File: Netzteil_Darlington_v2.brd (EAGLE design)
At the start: 141 x 115.5 mm, 169 parts, among them IC1 NCP718BSN330T1G, IC10 LT4320DIL08, IC11 OPA2197, IC12 REF5040, IC13 OPA2197, IC15 LD33V, IC17 7818TV, IC18 ADS1015, IC19 ADS1015, IC2 OPA2197, IC3 DAC8311, IC4 VXO78012-1000, IC5 7815TV, IC6 VXO7805-1000, IC7 DAC8311, IC8 LTC6102HMS8#PBF, IC9 NCP718BSN330T1G, T1 IRLL110TRPBF, T10 BC847ALT1G, T11 BC847ALT1G, T12 DMG2302UK-7, T13 DMG2302UK-7, T14 DMG2302UK-7, T2 BC847ALT1G, T3 BD139, T4 DMMT5551-7-F, T5 TIP3055, T6 TIP3055, T7 BD139

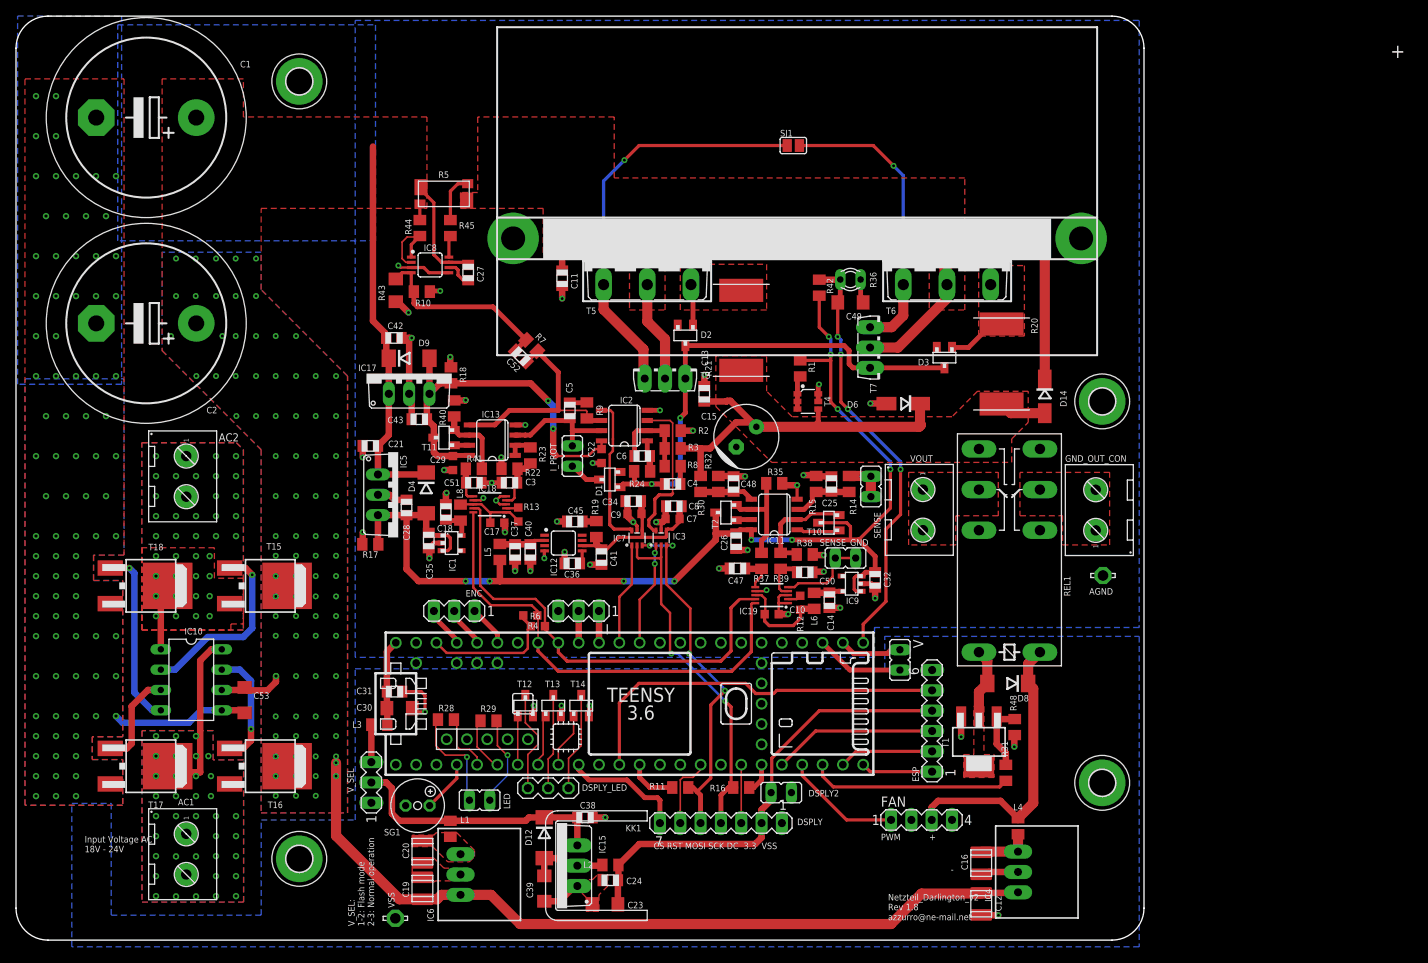
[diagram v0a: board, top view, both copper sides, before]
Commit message: Update to v1.9
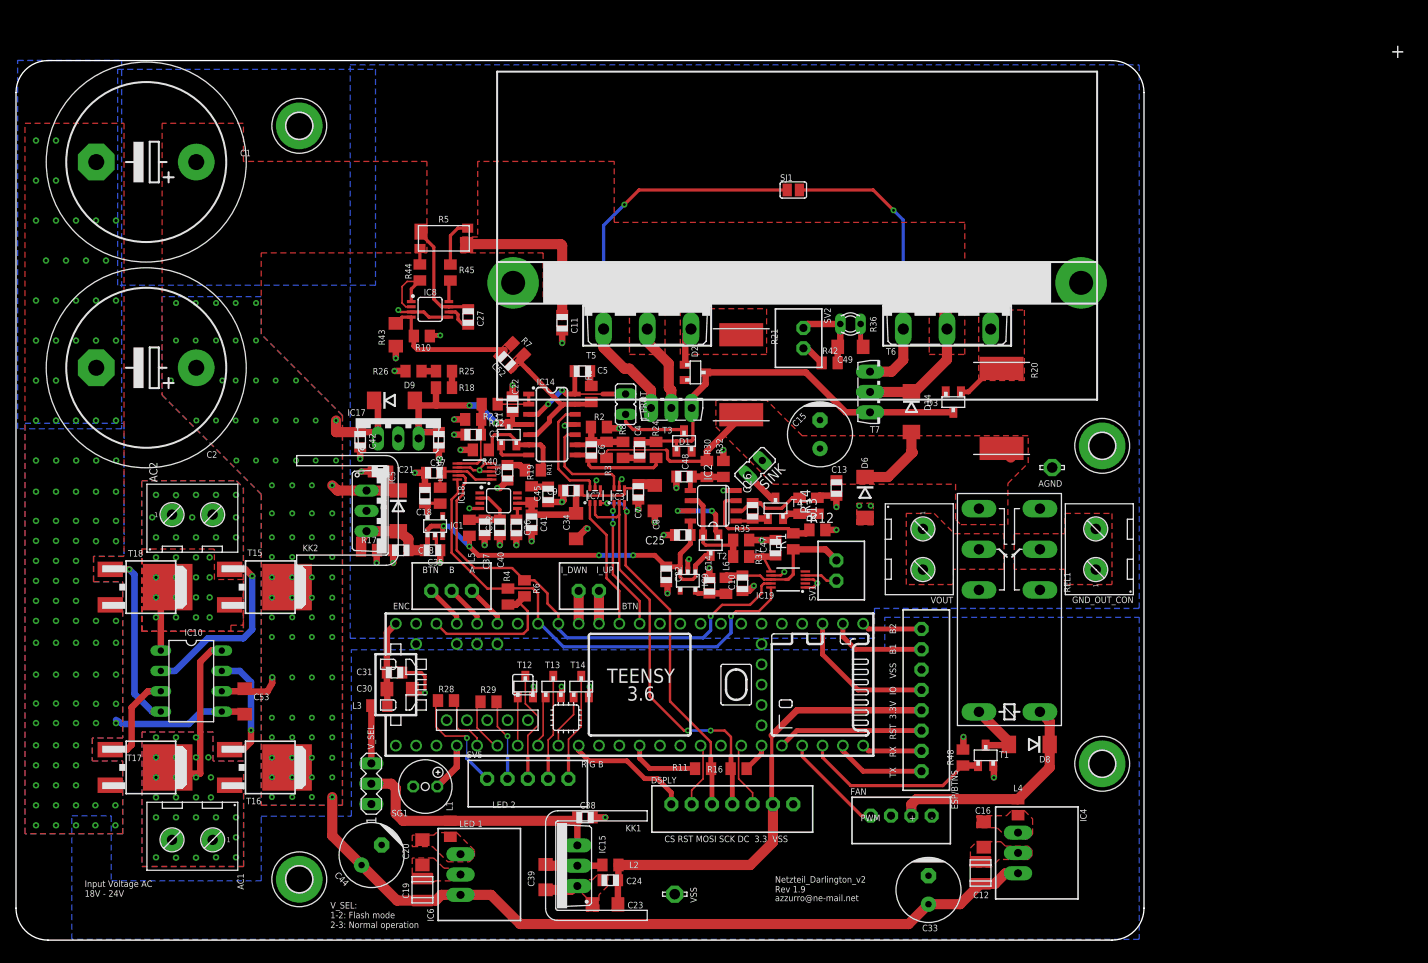
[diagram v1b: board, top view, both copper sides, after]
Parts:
- removed C29: 100n, goujine:C0603K
- removed C50: 10n, goujine:0805
- removed D12: 1N4007, diode:DO214AA
- removed DSPLY2, LED, SENSE, SENSE_GND, V: (no value), jumper:JP1
- removed DSPLY_LED: (no value), neumluc:MA03-1
- removed ESP: (no value), con-lstb:MA06-1
- removed I: (no value), con-lstb:MA03-1
- removed IC11, IC13: OPA2197, goujine:SOP8
- removed R15: 10.1k 0.1% RN732ATTD1012B25, neumluc:C0805K
- removed R31: 360R, neumluc:C0805K
- removed R38: 4.7k, neumluc:C0805K
- removed R39: 100R, neumluc:C0805K
- removed T10: BC847ALT1G, neumluc:SOT23-BEC
- added BTN, SV1, SV2: (no value), neumluc:JST-PH-2.0-2P
- added C33, C44: 100µ/50V, goujine:C+/3.5/8
- added ESP/BTNS: (no value), neumluc:JST-PH-2.0-8P
- added IC14: QUAD-OPVOPA4197, neumluc:SO14
- added KK2: D01S, heatsink:D01S
- added R25, R26: 1k 1% 1/8W, neumluc:C0805K
- added SINK: (no value), jumper:JP1
- added SV5: (no value), neumluc:JST-PH-2.0-5P
- C1, C2: value UVZ1H103MRD -> 10000µ/50V
- C10, C17, C7, C9: device goujine:C0603K -> goujine:0805
- C11: value 330n opt -> 330n opt/50V
- C13: value 100n opt -> 100n opt/50V
- C15: value 100µ/50V EEU-FR1H101 -> 100µ/50V
- C16: value 10µ/16V -> 10µ/25V; device we-rcl:C1210 -> goujine:1206
- C20: device we-rcl:C1210 -> goujine:1206
- C21, C42: value 330n -> 330n/50V
- C22: value 100n -> 100n/35V; device goujine:C0603K -> goujine:0805
- C23, C30, C39, C49: value 10µ / C3216X7R1E106M160AB -> 10µ/16V
- C24, C3, C31, C38, C48: value 100n -> 100n/16V
- C25, C28, C43: value 100n -> 100n/35V
- C26: value 100n -> 1n/50V
- C27: value 100n -> 100n/50V
- C32, C35, C37: value 1µ/50V -> 1µ/35V
- C34, C8: device goujine:0805 -> goujine:1206
- C4: value 10n -> 10n/50V
- C40: value 100n/50V -> 100n/35V
- C47, C51: value 10n -> 10n/16V
- C5: value 1n -> 1n/50V
- C52: value 22p opt -> 22p opt/35V C0G
- C53: value (none) -> 1µ/50V
- C6: value 22pF -> 22pF/35V C0G
- D14, D6: value CDBA5200-HF -> CGRB307-G; device neumluc:DO214AC-2 -> neumluc:DO214AA-CGRB307-G
- D4, D8, D9: value 1N4007 -> CGRB307-G; device diode:DO214AA -> neumluc:DO214AA-CGRB307-G
- DSPLY: device con-lstb:MA07-1 -> neumluc:JST-PH-2.0-7P
- ENC: device con-lstb:MA03-1 -> neumluc:JST-PH-2.0-3P
- FAN: device con-lstb:MA04-1 -> neumluc:JST-PH-2.0-4P
- IC18, IC19: value ADS1015 -> ADS1115; device SparkFun-IC-Conversion:MSOP10 -> neumluc:MSOP10
- IC2: value OPA2197 -> (none)
- R1: value 2k2 5% -> 12k 0.5% 50 ppm 1/10W
- R10: value 4.7k opt -> 4.7k opt 1% 1/10W
- R11, R16: value 22R -> 22R 5% 1/10W
- R12: value 10k -> 221R 0.5% 50ppm 1/10W; device neumluc:C0603K -> neumluc:C0805K
- R13: value 10k -> 1k 0.5% 50 ppm 1/10W; device neumluc:C0603K -> neumluc:C0805K
- R14: value 90.9k 0.1% RN73C2A90K9BTDF -> 10R 0.5% 50 ppm 1/4W
- R17: value 2k2 -> 2k2 5% 1/8W
- R18: value 2k2 -> 1k 1% 1/8W
- R19: value 1.27R -> 1.27R 1% 1/10W
- R20, R21: value 0R1 0.5% -> 0R1 0.5% 7W
- R22, R32: value 10.1k 0.1% RN732ATTD1012B25 -> 10.1k 0.1% 10ppm 1/10W
- R23, R30: value 90.9k 0.1% RN73C2A90K9BTDF -> 90.9k 0.1% 10ppm 1/10W
- R24: value 1k opt -> 1k 1% 1/10W
- R28, R29: value 220R -> 220R 5% 1/10W
- R35, R40: value 4.7k -> 4.7k 5% 1/10W
- R37: value 100R -> 2.2k 5% 1/8W
- R4, R6: value 10k -> 10k 5% 1/10W; device neumluc:C0603K -> neumluc:C0805K
- R41: value 100R -> 100R 5% 1/10W
- R42: value 390k 1% -> 65k 1% 1/10W
- R43: value 5k 0.1% low ppm TNPW12065K00BEEN -> 5k 0.1% 25ppm
- R44, R45: value 100R 0.1% low ppm PCF0805-13-100RBT1 -> 100R 0.1% 5ppm 1/10W
- R48, R7: value 10k -> 10k 5% 1/10W
- R5: value 10m -> 10m 0.1% 15ppm 0.5W
- R8: value 47k -> 47k 1% 1/10W
- R9: value 4.7k -> 4.7k 1% 1/10W
- T1: value IRLL110TRPBF -> PMV130ENEAR; device goujine:SOT223-4 -> neumluc:SOT23
- T12, T13, T14: value DMG2302UK-7 -> PMV130ENEAR
- T15, T16, T17, T18: value (none) -> IRFR7546TRPBF
- T4: value DMMT5551-7-F -> PMV130ENEAR; device neumluc:SOT-26 -> neumluc:SOT23
- moved R13 35.2 mm to (97.9, 54.3), turned to 270 degrees
- moved VSS 35.1 mm to (82.3, 5.74)
- moved C32 26.1 mm to (81.3, 45.7)
- moved R1 21.6 mm to (97.2, 49.8), turned to 90 degrees
- moved IC9 20.5 mm to (84.0, 44.9), turned to 180 degrees
- moved C13 20.3 mm to (102.6, 56.5), turned to 270 degrees
- moved C25 19.6 mm to (83.3, 50.6), turned to 180 degrees
- moved D14 16.8 mm to (111.9, 66.1)
- moved C14 15.1 mm to (86.7, 44.3), turned to 270 degrees
- moved IC2 15.0 mm to (87.2, 54.3)
- moved AGND 14.9 mm to (129.5, 59.1)
- moved T4 14.0 mm to (94.9, 54.0), turned to 0 degrees
- moved C42 13.4 mm to (43.0, 62.5), turned to 270 degrees
- moved C22 12.9 mm to (62.1, 67.0), turned to 90 degrees
- moved D6 12.7 mm to (106.1, 55.3), turned to 270 degrees
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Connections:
- removed net ADC_CH1: C50.1, IC19.4, R39.2
- removed net ADC_SENSE: C25.1, IC11.3, R14.1, R15.2
- removed net N$12: D8.A, REL1.+, T1.2, T1.4
- removed net N$37: R31.1, R48.2, T1.1
- removed net N$40: IC11.7, T2.B
- removed net N$42: IC11.1, T10.B
- removed net N$43: IC11.2, R38.1, R39.1, T10.E
- removed net N$44: IC13.7, T11.B
- removed net SENSE: R14.2, SENSE.1, SENSE.2
- removed net SENSE_GND: IC19.5, SENSE_GND.1, SENSE_GND.2
- new net 3.3V_A2_FILTERED: C10.1, IC19.8, L6.1, R1.1, SV1.2
- new net 3.3V_TH: R42.1, SV2.2
- new net N$26: R18.2, R25.1
- new net N$30: R25.2, R26.1
- new net N$31: C6.1, IC14.9, R2.2, R3.2, R8.2
- new net N$33: C26.1, IC2.1, T4.1
- new net N$34: SINK.2, T4.3
- new net N$38: D8.A, REL1.+, T1.3
- new net TH0_ADC: IC19.4, SV1.1
- net +15V: now also C25.1, IC2.8; no longer C26.1, IC11.8, R1.1, R42.1, T10.C
- net +18V: now also IC14.4; no longer C29.1, IC13.8, IC2.8
- net +27V: now also C33.+, C44.+
- net +3.3V: now also DSPLY.6, ESP/BTNS.4; no longer DSPLY.2, DSPLY2.2, ESP.4
- net +5V_INT_D: no longer D12.C
- net +V_ADJ: now also SINK.1; no longer T4.4
- net ADC_CH0: now also IC18.4; no longer IC18.6
- net ADC_CH3: now also IC18.6; no longer IC18.4
- net ADC_VOUT: now also IC2.5; no longer IC11.5
- net AGND: now also IC14.11, R12.2, R14.2, R26.2, U$33.GND2; no longer C26.2, C29.2, C50.2, I.3, IC11.4, IC13.4, R15.1, R18.2, R38.2, T4.5, T4.6
- net BTN_I_DOWN: now also BTN.2; no longer I.2
- net BTN_I_UP: now also BTN.1; no longer I.1
- net BTN_V_DOWN: now also ESP/BTNS.8, U$33.33/A14; no longer U$33.35/A16, V.2
- net BTN_V_UP: now also ESP/BTNS.7; no longer V.1
- net CRNT_READ: now also IC14.13, IC14.5; no longer IC13.5, IC2.6
- net DSPLY_CS: now also DSPLY.1; no longer DSPLY.7
- net DSPLY_DC: now also DSPLY.5; no longer DSPLY.3
- net DSPLY_RST: now also DSPLY.2; no longer DSPLY.6
- net ESP-IO: now also ESP/BTNS.5, U$33.35/A16; no longer ESP.5, U$33.10/CS
- net ESP-RST: now also ESP/BTNS.3; no longer ESP.3
- net ESP-RX: now also ESP/BTNS.2, U$33.32/A13; no longer ESP.2, U$33.31/A12
- net ESP-TX: now also ESP/BTNS.1, U$33.31/A12; no longer ESP.1, U$33.32/A13
- net ISET: now also IC14.12; no longer IC2.5
- net MOSI: now also DSPLY.3; no longer DSPLY.5
- net N$11: now also IC2.3, R12.1; no longer T4.1, T4.2, T4.3
- net N$16: now also R14.1, T4.2; no longer IC18.2
- net N$18: now also C26.2, IC2.2, R13.1; no longer IC19.2, R12.2
- net N$19: now also IC2.7, T2.B; no longer C10.1, IC19.8, L6.1, R12.1
- net N$20: now also SV5.1; no longer LED.1
- net N$21: now also IC14.8; no longer IC2.1
- net N$23: now also SV5.2; no longer LED.2
- net N$24: no longer R13.1
- net N$35: no longer D12.A
- net N$41: now also IC2.6; no longer IC11.6
- net N$45: now also IC14.6; no longer IC13.6
- net N$46: now also SV5.4; no longer DSPLY_LED.2
- net N$48: now also SV5.5; no longer DSPLY_LED.3
- net N$6: now also IC14.7, T11.B; no longer C6.1, IC2.2, R2.2, R3.2, R8.2
- net N$7: now also SV5.3; no longer DSPLY_LED.1
- net OVRCRNT_DET: now also IC14.14, IC14.3; no longer IC13.3, IC2.7
- net OVRCRNT_DET_BUF: now also IC14.1, IC14.2; no longer IC13.1, IC13.2
- net REL-OUT: now also R48.2, T1.1; no longer R31.2
- net TH0: now also SV2.1; no longer U$33.33/A14
- net VSET: now also IC14.10; no longer IC2.3
- net VSS: now also C33.-, C44.-, DSPLY.7, ESP/BTNS.6, T1.2; no longer DSPLY.1, DSPLY2.1, ESP.6, T1.3
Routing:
- net +15V: track 147.4 -> 65.7 mm, vias 10 -> 4
- net TH0: track 53.4 -> 9.82 mm, vias 4 -> 0
- net ESP-IO: track 49.1 -> 18.1 mm
- net +27V: track 173.2 -> 144.7 mm
- net +V_ADJ: track 61.2 -> 33.7 mm
- net +18V: track 48.3 -> 28.6 mm
- net AGND: track 107.8 -> 89.3 mm, vias 44 -> 46
- net 3.3V_A2_FILTERED: track 0.00 -> 18.2 mm
- net N$43: track 13.6 -> 0.00 mm
- net N$22: track 63.1 -> 50.8 mm, vias 2 -> 0
- net N$11: track 4.22 -> 15.6 mm
- net SENSE_GND: track 11.1 -> 0.00 mm
- net N$3: track 70.3 -> 59.3 mm
- net CRNT_READ: track 28.7 -> 18.7 mm
- net N$12: track 8.91 -> 0.00 mm
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- added copper zone on layer 1, net AGND
- added copper zone on layer 1, net CRNT_READ
- added copper zone on layer 1, net CRNT_READ_RAW
- added copper zone on layer 1, net N$13
- removed copper zone on layer 1, net N$12
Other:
- board size 141 x 115.5 mm -> 141 x 109.9 mm
- board text added: "3.3V"
- board text added: "A"
- board text added: "B"
- board text added: "B1"
- board text added: "B2"
- board text added: "BTN"
- board text added: "IO"
- board text added: "I_DWN"
- board text added: "I_UP"
- board text added: "LED 1"
- board text added: "LED 2"
- board text added: "Netzteil_Darlington_v2 Rev 1.9"
- board text added: "R G B"
- board text added: "RST"
- board text added: "RX"
- board text added: "TX"
- board text added: "VSS"
- board text removed: "Netzteil_Darlington_v2 Rev 1.8"
